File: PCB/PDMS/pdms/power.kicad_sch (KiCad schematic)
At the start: 32 parts, among them IC10 LDO40LPU50RY, IC11 MP2332HGTL-P, IC14 LDO40LPU50RY, IC3 LDO40LPU33RY, Q1 AO3401A, Q11 AO3401A

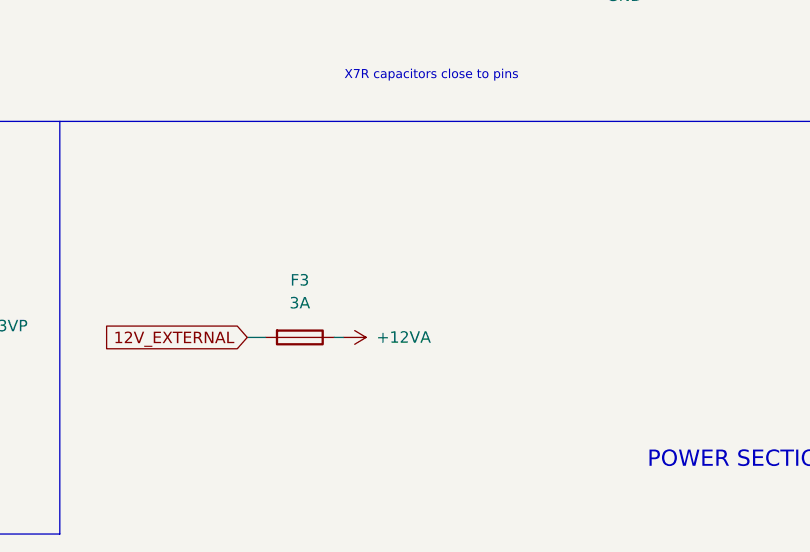
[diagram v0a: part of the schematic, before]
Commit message: Finished 2024 version + gerbers
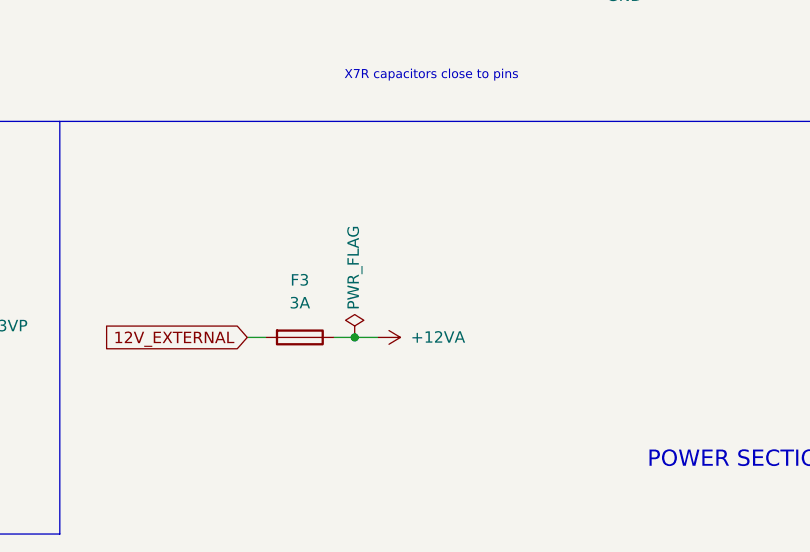
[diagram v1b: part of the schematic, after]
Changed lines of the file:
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@@
   (junction (at 94.615 42.545) (diameter 0) (color 0 0 0 0)
+  )
+  (junction (at 154.813 175.768) (diameter 0) (color 0 0 0 0)
   )
   (junction (at 149.225 45.72) (diameter 0) (color 0 0 0 0)
@@
     (stroke (width 0) (type default) (color 0 0 0 0))
   )
+  (wire (pts (xy 154.813 175.768) (xy 152.527 175.768))
+    (stroke (width 0) (type default) (color 0 0 0 0))
+  )
   (wire (pts (xy 215.265 49.53) (xy 215.265 45.72))
     (stroke (width 0) (type default) (color 0 0 0 0))
@@
     (stroke (width 0) (type default) (color 0 0 0 0))
   )
-  (wire (pts (xy 153.543 175.768) (xy 152.527 175.768))
+  (wire (pts (xy 157.353 175.768) (xy 154.813 175.768))
     (stroke (width 0) (type default) (color 0 0 0 0))
   )
@@
     (pin "1")
   )
-  (symbol (lib_id "power:+12VA") (at 153.543 175.768 270) (unit 1)
-    (in_bom yes) (on_board yes) (fields_autoplaced)
-    (property "Reference" "#PWR0136" (id 0) (at 149.733 175.768 0)
-      (effects (font (size 1.27 1.27)) hide)
-    )
-    (property "Value" "+12VA" (id 1) (at 157.226 175.7679 90)
-      (effects (font (size 1.27 1.27)) (justify left))
-    )
-    (property "Footprint" "" (id 2) (at 153.543 175.768 0)
-      (effects (font (size 1.27 1.27)) hide)
-    )
-    (property "Datasheet" "" (id 3) (at 153.543 175.768 0)
+  (symbol (lib_id "power:+12VA") (at 157.353 175.768 270) (unit 1)
+    (in_bom yes) (on_board yes) (fields_autoplaced)
+    (property "Reference" "#PWR0136" (id 0) (at 153.543 175.768 0)
+      (effects (font (size 1.27 1.27)) hide)
+    )
+    (property "Value" "+12VA" (id 1) (at 161.036 175.7679 90)
+      (effects (font (size 1.27 1.27)) (justify left))
+    )
+    (property "Footprint" "" (id 2) (at 157.353 175.768 0)
+      (effects (font (size 1.27 1.27)) hide)
+    )
+    (property "Datasheet" "" (id 3) (at 157.353 175.768 0)
       (effects (font (size 1.27 1.27)) hide)
     )
@@
       (effects (font (size 1.27 1.27)) hide)
     )
+    (pin "1")
+  )
+  (symbol (lib_id "power:PWR_FLAG") (at 154.813 175.768 0) (unit 1)
+    (in_bom yes) (on_board yes)
+    (property "Reference" "#FLG0108" (id 0) (at 154.813 173.863 0)
+      (effects (font (size 1.27 1.27)) hide)
+    )
+    (property "Value" "PWR_FLAG" (id 1) (at 154.686 168.021 90))
+    (property "Footprint" "" (id 2) (at 154.813 175.768 0)
+      (effects (font (size 1.27 1.27)) hide)
+    )
+    (property "Datasheet" "~" (id 3) (at 154.813 175.768 0)
+      (effects (font (size 1.27 1.27)) hide)
+    )
